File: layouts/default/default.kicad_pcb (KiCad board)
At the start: 2 copper layers, 27.1 x 34.7 mm, 18 parts

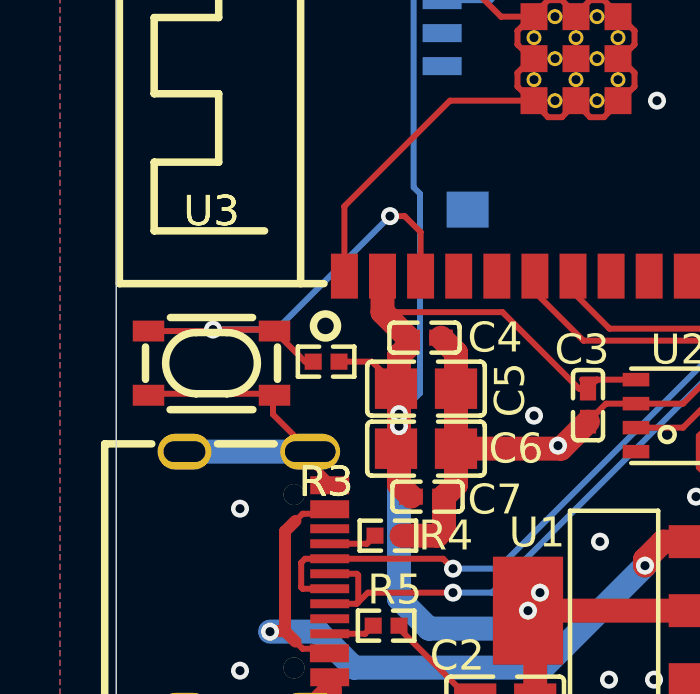
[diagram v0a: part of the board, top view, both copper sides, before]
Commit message: updated button
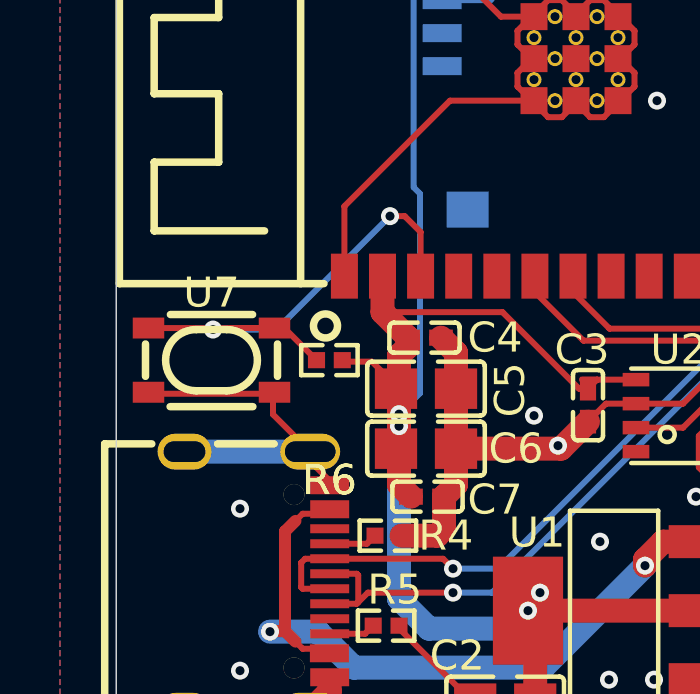
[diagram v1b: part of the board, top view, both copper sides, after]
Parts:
- removed R3: 10kΩ ±1% 62.5mW, atopile:R0402-56259e
- removed U3: , lib:KEY-SMD_4P-L4.2-W3.2-P2.20-LS4.6
- added R6: 10kΩ ±1% 62.5mW, atopile:R0402-56259e, F.Cu at (77.2, 82.2)
- added U7: , lib:KEY-SMD_4P-L4.2-W3.2-P2.20-LS4.6, F.Cu at (73.2, 82.2)
- C1, C2: value 10µF ±10% 25V X5R -> 100nF ±10% 50V X7R
- R1, R2: value 1kΩ ±1% 62.5mW -> 10kΩ ±1% 62.5mW
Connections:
- C1 pad 1: hv -> hv-1
- C2 pad 1: hv-1 -> hv
- C3 pad 1: hv-1 -> hv
- C4 pad 1: hv-1 -> hv
- C5 pad 1: hv-1 -> hv
- C6 pad 1: hv-1 -> hv
- C7 pad 1: hv-1 -> hv
- U1 pad 2: hv-1 -> hv
- U1 pad 3: hv -> hv-1
- U1 pad 4: hv-1 -> hv
- U2 pad 8: hv-1 -> hv
- U4 pad 2: hv-1 -> hv
- U4 pad 3: in -> EN
- U5 pad A4: hv -> hv-1
- U5 pad A9: hv -> hv-1
- U5 pad B4: hv -> hv-1
- U5 pad B9: hv -> hv-1
- U6 pad 4: hv-1 -> hv
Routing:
- net hv-1: track 58.7 -> 27.3 mm, vias 4 -> 2
- net hv: track 27.3 -> 58.7 mm, vias 2 -> 4
- net in: track 16.4 -> 18.7 mm
